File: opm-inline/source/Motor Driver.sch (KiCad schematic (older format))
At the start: 38 parts, among them IC1 TMC6200-TA, Q1 YJG95G06A, Q2 YJG95G06A, Q3 YJG95G06A, Q4 YJG95G06A, Q5 YJG95G06A, Q6 YJG95G06A

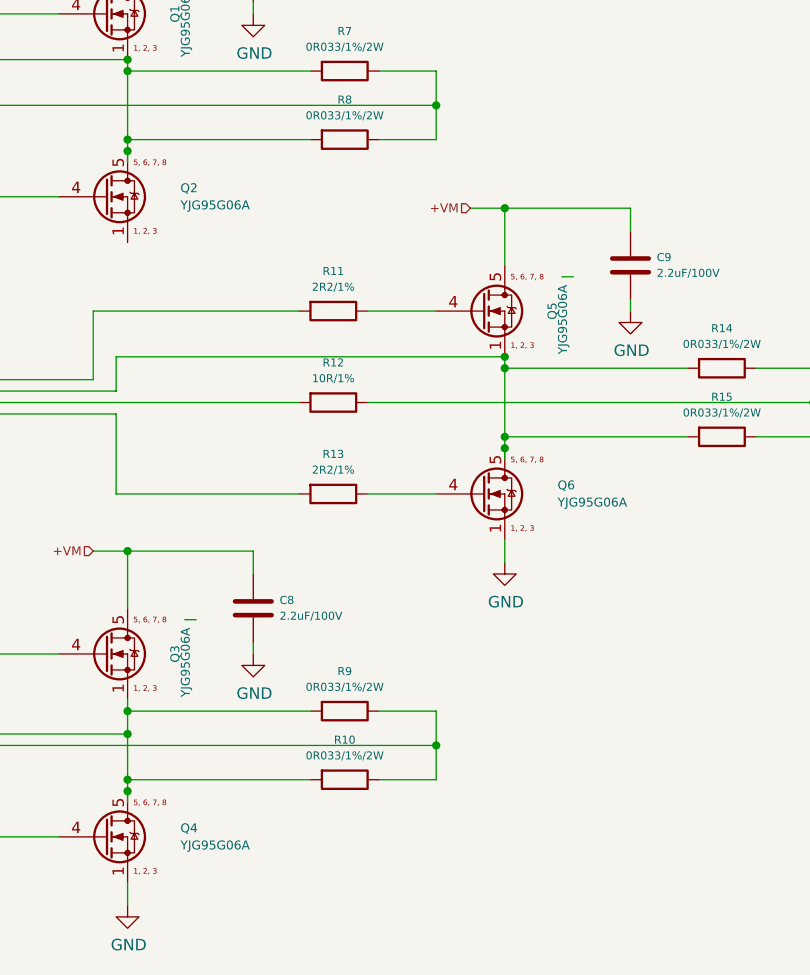
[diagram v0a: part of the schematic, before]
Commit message: cleanup
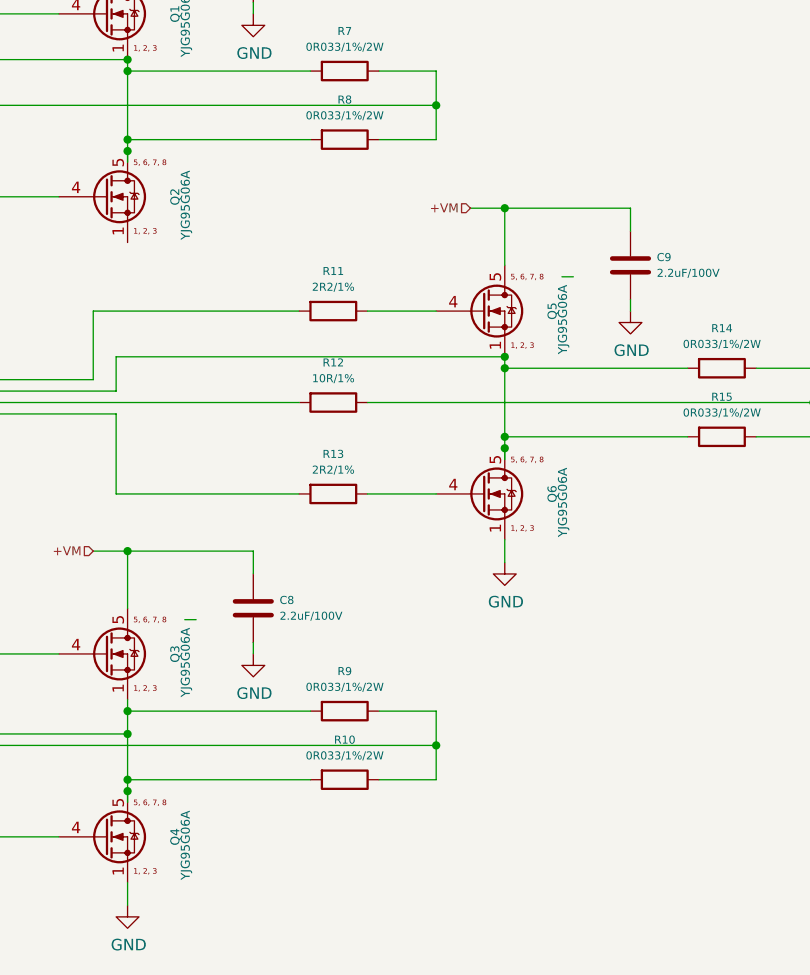
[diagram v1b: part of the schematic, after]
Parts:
- R10, R14, R15, R7, R8, R9: LCSC C2688862 -> C2838960; manf_num BVS-I-R003-1.0 -> LMP25NF2P0R033
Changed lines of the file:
@@
 AR Path="/61C4FD8F" Ref="Q4"  Part="1"
 AR Path="/5D5FDD98/61C4FD8F" Ref="Q4"  Part="1"
-F 0 "Q4" H 8031 5988 39  0000 L CNN
-F 1 "YJG95G06A" H 8031 5913 39  0000 L CNN
+F 0 "Q4" V 8031 5988 39  0000 R BNN
+F 1 "YJG95G06A" V 8031 5913 39  0000 C TNN
 F 2 "Package_TO_SOT_SMD:TDSON-8-1" H 7900 5875 39  0001 L CIN
 F 3 "" V 7700 5950 50  0001 L CNN
@@
 F 1 "0R033/1%/2W" V 8645 5400 35  0000 C CNN
 F 2 "Resistor_SMD:R_0603_1608Metric" V 8680 5400 50  0001 C CNN
-F 3 "https://www.isabellenhuette.de/fileadmin/Daten/Praezisionswiderstaende/Datenblaetter/BVT.PDF" H 8750 5400 50  0001 C CNN
-F 4 "C2688862" V 8750 5400 50  0001 C CNN "LCSC"
-F 5 "BVS-I-R003-1.0" V 8750 5400 50  0001 C CNN "manf_num"
+F 3 "https://datasheet.lcsc.com/lcsc/2108141930_prosemi-LMP25NF2P0R033_C2838960.pdf" H 8750 5400 50  0001 C CNN
+F 4 "C2838960" V 8750 5400 50  0001 C CNN "LCSC"
+F 5 "LMP25NF2P0R033" V 8750 5400 50  0001 C CNN "manf_num"
 	1    8750 5400
 	0    1    1    0
@@
 F 1 "0R033/1%/2W" V 8645 5700 35  0000 C CNN
 F 2 "Resistor_SMD:R_0603_1608Metric" V 8680 5700 50  0001 C CNN
-F 3 "https://www.isabellenhuette.de/fileadmin/Daten/Praezisionswiderstaende/Datenblaetter/BVT.PDF" H 8750 5700 50  0001 C CNN
-F 4 "C2688862" V 8750 5700 50  0001 C CNN "LCSC"
-F 5 "BVS-I-R003-1.0" V 8750 5700 50  0001 C CNN "manf_num"
+F 3 "https://datasheet.lcsc.com/lcsc/2108141930_prosemi-LMP25NF2P0R033_C2838960.pdf" H 8750 5700 50  0001 C CNN
+F 4 "C2838960" V 8750 5700 50  0001 C CNN "LCSC"
+F 5 "LMP25NF2P0R033" V 8750 5700 50  0001 C CNN "manf_num"
 	1    8750 5700
 	0    1    1    0
@@
 AR Path="/61D8AF0A" Ref="Q6"  Part="1"
 AR Path="/5D5FDD98/61D8AF0A" Ref="Q6"  Part="1"
-F 0 "Q6" H 9681 4488 39  0000 L CNN
-F 1 "YJG95G06A" H 9681 4413 39  0000 L CNN
+F 0 "Q6" V 9681 4488 39  0000 R BNN
+F 1 "YJG95G06A" V 9681 4413 39  0000 C TNN
 F 2 "Package_TO_SOT_SMD:TDSON-8-1" H 9550 4375 39  0001 L CIN
 F 3 "" V 9350 4450 50  0001 L CNN
@@
 F 1 "0R033/1%/2W" V 10295 3900 35  0000 C CNN
 F 2 "Resistor_SMD:R_0603_1608Metric" V 10330 3900 50  0001 C CNN
-F 3 "https://www.isabellenhuette.de/fileadmin/Daten/Praezisionswiderstaende/Datenblaetter/BVT.PDF" H 10400 3900 50  0001 C CNN
-F 4 "C2688862" V 10400 3900 50  0001 C CNN "LCSC"
-F 5 "BVS-I-R003-1.0" V 10400 3900 50  0001 C CNN "manf_num"
+F 3 "https://datasheet.lcsc.com/lcsc/2108141930_prosemi-LMP25NF2P0R033_C2838960.pdf" H 10400 3900 50  0001 C CNN
+F 4 "C2838960" V 10400 3900 50  0001 C CNN "LCSC"
+F 5 "LMP25NF2P0R033" V 10400 3900 50  0001 C CNN "manf_num"
 	1    10400 3900
 	0    1    1    0
@@
 F 1 "0R033/1%/2W" V 10295 4200 35  0000 C CNN
 F 2 "Resistor_SMD:R_0603_1608Metric" V 10330 4200 50  0001 C CNN
-F 3 "https://www.isabellenhuette.de/fileadmin/Daten/Praezisionswiderstaende/Datenblaetter/BVT.PDF" H 10400 4200 50  0001 C CNN
-F 4 "C2688862" V 10400 4200 50  0001 C CNN "LCSC"
-F 5 "BVS-I-R003-1.0" V 10400 4200 50  0001 C CNN "manf_num"
+F 3 "https://datasheet.lcsc.com/lcsc/2108141930_prosemi-LMP25NF2P0R033_C2838960.pdf" H 10400 4200 50  0001 C CNN
+F 4 "C2838960" V 10400 4200 50  0001 C CNN "LCSC"
+F 5 "LMP25NF2P0R033" V 10400 4200 50  0001 C CNN "manf_num"
 	1    10400 4200
 	0    1    1    0
@@
 AR Path="/61D9B6B4" Ref="Q2"  Part="1"
 AR Path="/5D5FDD98/61D9B6B4" Ref="Q2"  Part="1"
-F 0 "Q2" H 8031 3188 39  0000 L CNN
-F 1 "YJG95G06A" H 8031 3113 39  0000 L CNN
+F 0 "Q2" V 8031 3188 39  0000 R BNN
+F 1 "YJG95G06A" V 8031 3113 39  0000 C TNN
 F 2 "Package_TO_SOT_SMD:TDSON-8-1" H 7900 3075 39  0001 L CIN
 F 3 "" V 7700 3150 50  0001 L CNN
@@
 F 1 "0R033/1%/2W" V 8645 2600 35  0000 C CNN
 F 2 "Resistor_SMD:R_0603_1608Metric" V 8680 2600 50  0001 C CNN
-F 3 "https://www.isabellenhuette.de/fileadmin/Daten/Praezisionswiderstaende/Datenblaetter/BVT.PDF" H 8750 2600 50  0001 C CNN
-F 4 "C2688862" V 8750 2600 50  0001 C CNN "LCSC"
-F 5 "BVS-I-R003-1.0" V 8750 2600 50  0001 C CNN "manf_num"
+F 3 "https://datasheet.lcsc.com/lcsc/2108141930_prosemi-LMP25NF2P0R033_C2838960.pdf" H 8750 2600 50  0001 C CNN
+F 4 "C2838960" V 8750 2600 50  0001 C CNN "LCSC"
+F 5 "LMP25NF2P0R033" V 8750 2600 50  0001 C CNN "manf_num"
 	1    8750 2600
 	0    1    1    0
@@
 F 1 "0R033/1%/2W" V 8645 2900 35  0000 C CNN
 F 2 "Resistor_SMD:R_0603_1608Metric" V 8680 2900 50  0001 C CNN
-F 3 "https://www.isabellenhuette.de/fileadmin/Daten/Praezisionswiderstaende/Datenblaetter/BVT.PDF" H 8750 2900 50  0001 C CNN
-F 4 "C2688862" V 8750 2900 50  0001 C CNN "LCSC"
-F 5 "BVS-I-R003-1.0" V 8750 2900 50  0001 C CNN "manf_num"
+F 3 "https://datasheet.lcsc.com/lcsc/2108141930_prosemi-LMP25NF2P0R033_C2838960.pdf" H 8750 2900 50  0001 C CNN
+F 4 "C2838960" V 8750 2900 50  0001 C CNN "LCSC"
+F 5 "LMP25NF2P0R033" V 8750 2900 50  0001 C CNN "manf_num"
 	1    8750 2900
 	0    1    1    0
